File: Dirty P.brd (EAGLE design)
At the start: 84.4 x 73.3 mm, 29 parts, among them SW1 FOOT_SW, SW2 108-0020-EVX, U1 MMBT3906, U2 MMBT3906, U3 MMBT3906

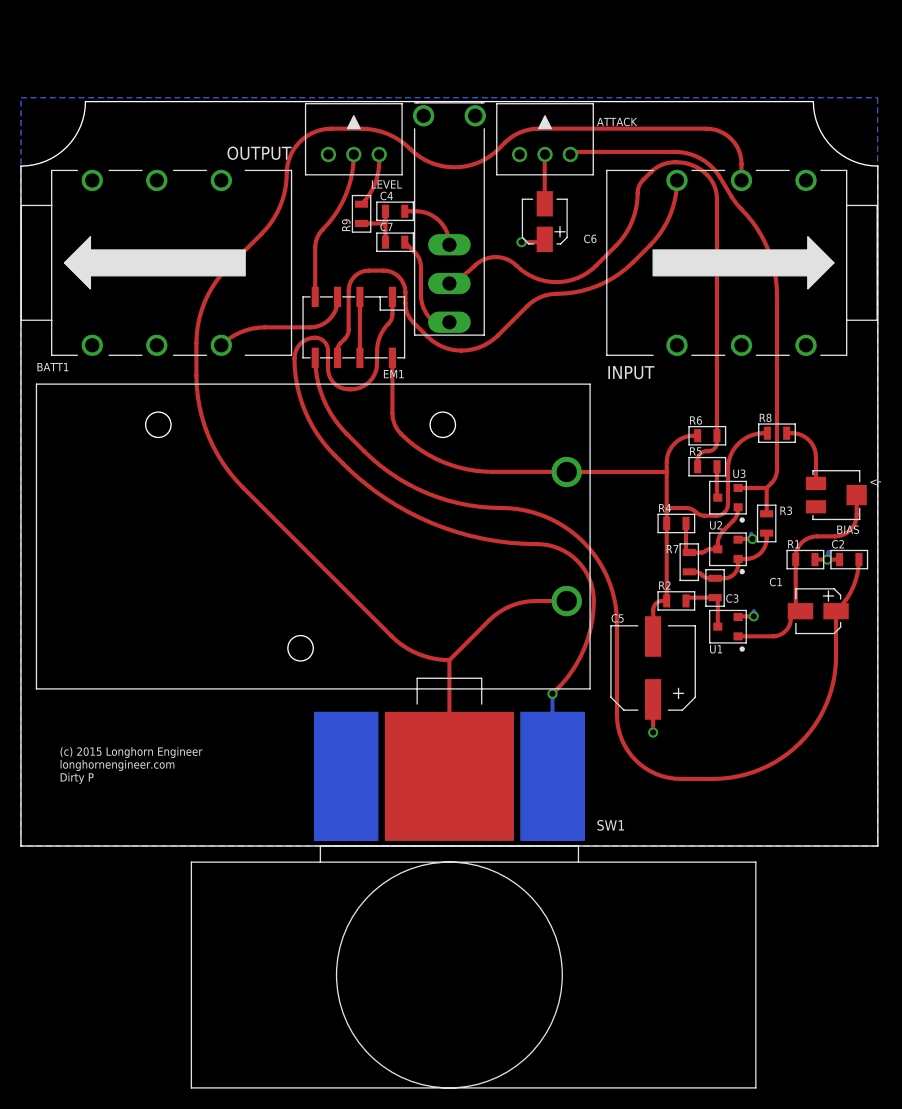
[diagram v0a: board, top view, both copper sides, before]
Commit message: Rev 3 Complete.
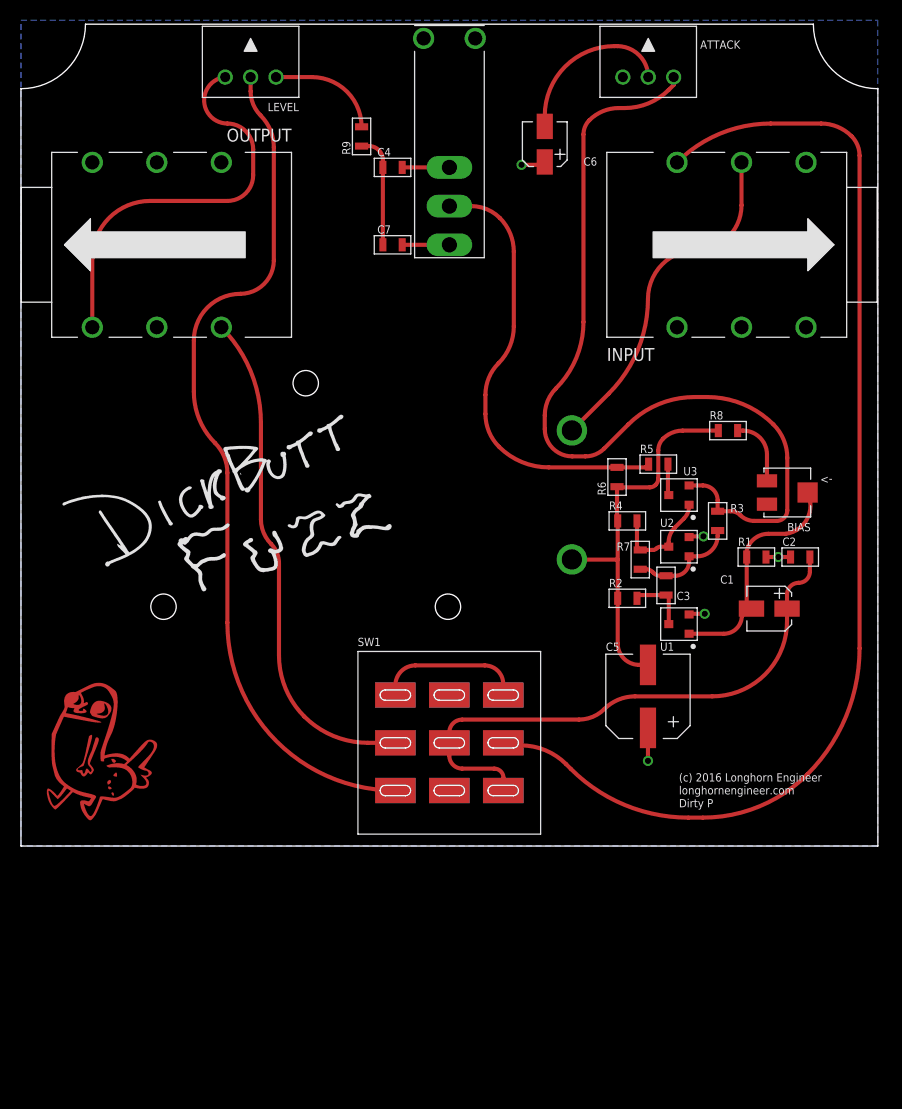
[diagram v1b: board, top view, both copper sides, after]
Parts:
- removed EM1: 6-1462037-4, PP_Electromechanical:IM_RELAY
- added U$2: DB_LOGO_COPPER_MEDIUM, PP_Aesthetics:DB_COPPER_MEDIUM
- SW1: value FOOT_SW -> (none); device PP_Electromechanical:FOOT_SW -> PP_Electromechanical:STOMPBOX_SW
- moved U$1 61.0 mm to (64.8, 1.27)
- moved BATT1 25.9 mm to (2.03, 19.6), flipped to the bottom, turned to 180 degrees
- moved ATTACK 12.7 mm to (61.7, 75.7)
- moved LEVEL 12.7 mm to (22.6, 75.7)
- moved SW1 10.2 mm to (42.2, 10.2), turned to 180 degrees
- moved R6 9.77 mm to (58.7, 36.3), turned to 90 degrees
- moved SW2 7.62 mm to (42.2, 66.8)
- moved R9 7.62 mm to (33.5, 69.8)
- moved C6 7.62 mm to (51.6, 69.1)
- moved C1 4.83 mm to (73.7, 23.4)
- moved C2 4.83 mm to (76.7, 28.4)
- moved R2 4.83 mm to (59.7, 24.4)
- moved R3 4.83 mm to (68.6, 32.0)
- moved R4 4.83 mm to (59.7, 32.0)
- moved U1 4.83 mm to (64.8, 21.8)
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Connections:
- removed net N$21: EM1.P$1, SW1.1
- net 9V: no longer SW1.COM
- net GND: now also SW1.B3, SW1.B6
- net N$11: now also SW1.C2, SW1.C5; no longer EM1.P$3
- net N$14: now also SW1.A1, SW1.A4, SW1.B2, SW1.B5; no longer EM1.P$5
- net N$17: now also SW1.A3, SW1.A6, SW1.C3, SW1.C6; no longer EM1.P$2, EM1.P$7
- net N$19: now also SW1.C1, SW1.C4; no longer EM1.P$4
- net N$4: no longer EM1.P$8
- net SIG_IN: now also SW1.A2, SW1.A5; no longer EM1.P$6
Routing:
- net 9V: track 136.8 -> 32.5 mm
- net N$21: track 78.3 -> 0.00 mm, vias 1 -> 0
- net N$19: track 14.8 -> 81.5 mm
- net SIG_IN: track 51.4 -> 115.6 mm
- net N$14: track 90.8 -> 54.3 mm
- net N$11: track 13.1 -> 49.4 mm
- net GND: track 13.0 -> 47.9 mm
- net N$4: track 72.4 -> 38.0 mm
- net N$8: track 54.4 -> 87.7 mm
- net N$5: track 61.6 -> 44.1 mm
- net N$9: track 5.07 -> 15.3 mm
- net N$17: track 6.00 -> 14.2 mm
- net N$16: track 10.2 -> 4.65 mm
- net N$13: track 5.48 -> 11.0 mm
- net N$10: track 5.24 -> 10.4 mm
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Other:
- board size 84.4 x 73.3 mm -> 84.4 x 80.9 mm
